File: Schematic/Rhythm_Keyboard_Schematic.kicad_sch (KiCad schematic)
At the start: 4 parts, among them U5 8080A, U5 8224, Y1 Crystal

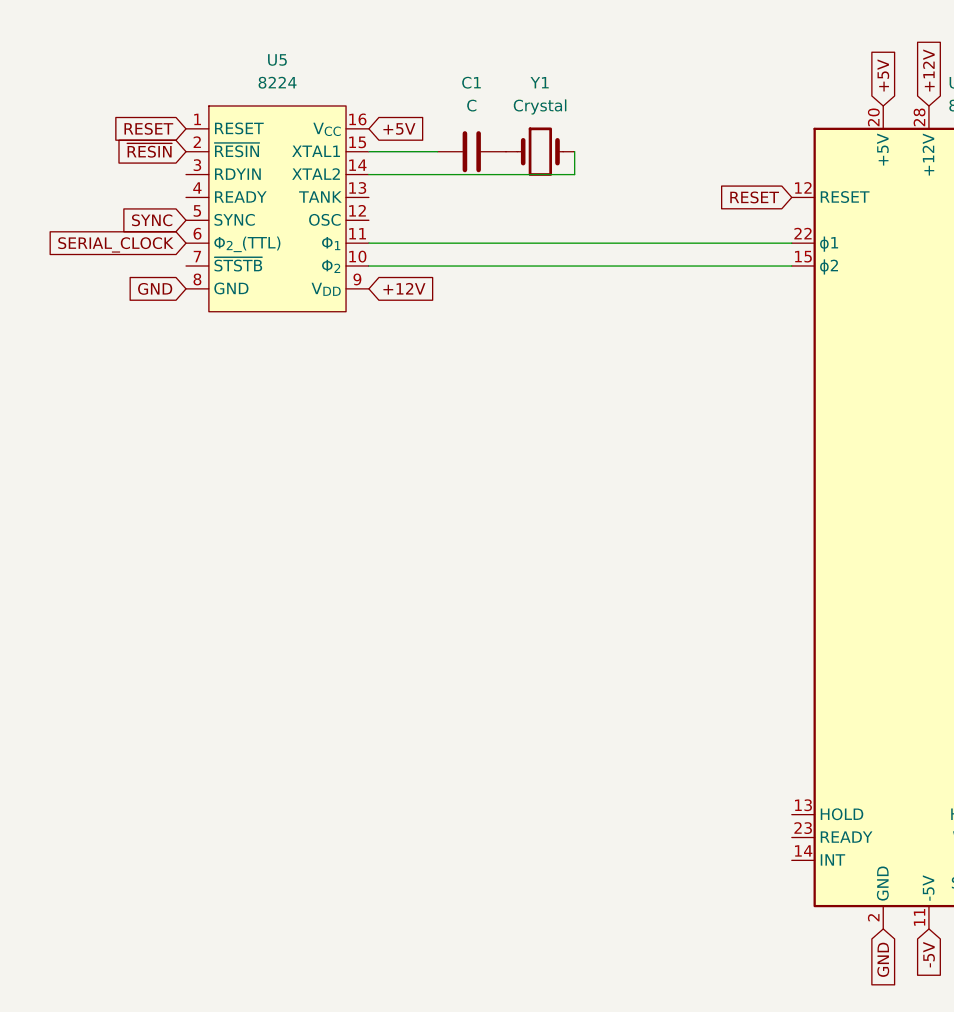
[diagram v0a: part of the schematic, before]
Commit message: Turning into a real schematic ...
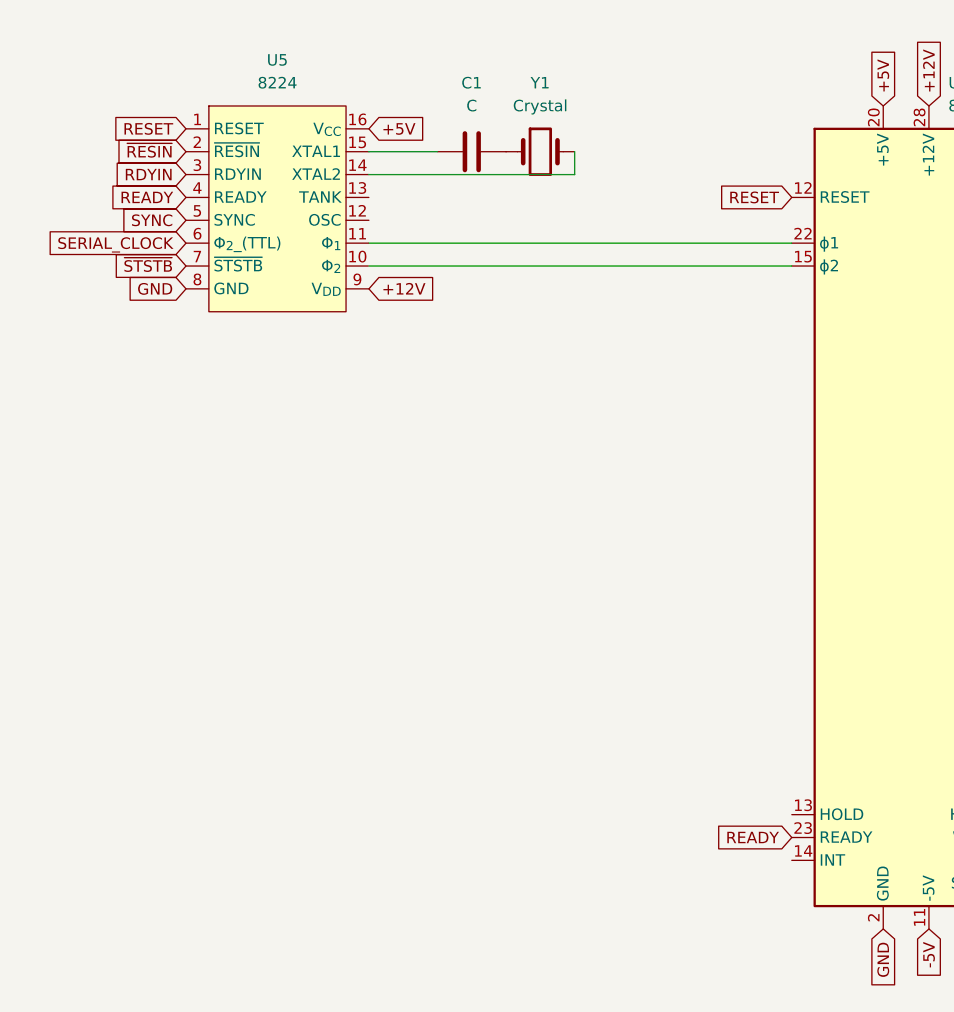
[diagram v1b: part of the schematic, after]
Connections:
- net RDYIN: now reaches U5.3 (RDYIN)
- net READY: now reaches U5.4 (READY)
- net READY: now also U5.23 (READY)
- net ~{STSTB}: now reaches U5.7 (~{STSTB})
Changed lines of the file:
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@@
+		)
+	)
+	(global_label "RDYIN"
+		(shape input)
+		(at 31.75 105.41 180)
+		(fields_autoplaced yes)
+		(effects
+			(font
+				(size 1.27 1.27)
+			)
+			(justify right)
+		)
+		(property "Intersheetrefs" "${INTERSHEET_REFS}"
+			(at 23.2009 105.41 0)
+			(effects
+				(font
+					(size 1.27 1.27)
+				)
+				(justify right)
+				(hide yes)
+			)
 		)
 	)
@@
 		)
 	)
+	(global_label "READY"
+		(shape input)
+		(at 31.75 107.95 180)
+		(fields_autoplaced yes)
+		(effects
+			(font
+				(size 1.27 1.27)
+			)
+			(justify right)
+		)
+		(property "Intersheetrefs" "${INTERSHEET_REFS}"
+			(at 22.8986 107.95 0)
+			(effects
+				(font
+					(size 1.27 1.27)
+				)
+				(justify right)
+				(hide yes)
+			)
+		)
+	)
 	(global_label "D3"
 		(shape input)
@@
 		)
 	)
+	(global_label "~{STSTB}"
+		(shape input)
+		(at 31.75 115.57 180)
+		(fields_autoplaced yes)
+		(effects
+			(font
+				(size 1.27 1.27)
+			)
+			(justify right)
+		)
+		(property "Intersheetrefs" "${INTERSHEET_REFS}"
+			(at 23.1406 115.57 0)
+			(effects
+				(font
+					(size 1.27 1.27)
+				)
+				(justify right)
+				(hide yes)
+			)
+		)
+	)
 	(global_label "DBIN"
 		(shape input)
@@
 				(hide yes)
 			)
+		)
+	)
+	(global_label "READY"
+		(shape input)
+		(at 99.06 179.07 180)
+		(fields_autoplaced yes)
+		(effects
+			(font
+				(size 1.27 1.27)
+			)
+			(justify right)
+		)
+		(property "Intersheetrefs" "${INTERSHEET_REFS}"
+			(at 90.2086 179.07 0)
+			(effects
+				(font
+					(size 1.27 1.27)
+				)
+				(justify right)
+				(hide yes)
+			)
